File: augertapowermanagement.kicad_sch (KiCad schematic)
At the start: 37 parts, among them J1 5v block, J10 USB_A_Stacked, J11 USB_A_Stacked, J12 USB_A_Stacked, J2 Image shown is a representati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, J3 gnd block, J4 0ZCF0200AF2C, J5 Screw_Terminal_01x10, J6 Screw_Terminal_01x10, J7 Screw_Terminal_01x10, J8 Screw_Terminal_01x08, J9 USB_A_Stacked, K1 J107F1CS203VDC.80, K2 J107F1CS203VDC.80, Q1 2N3904, SW1 SW_SPDT, U1 ESP32-DEVKITC-32D, U2 MCP9808_MSOP, U25 L7812

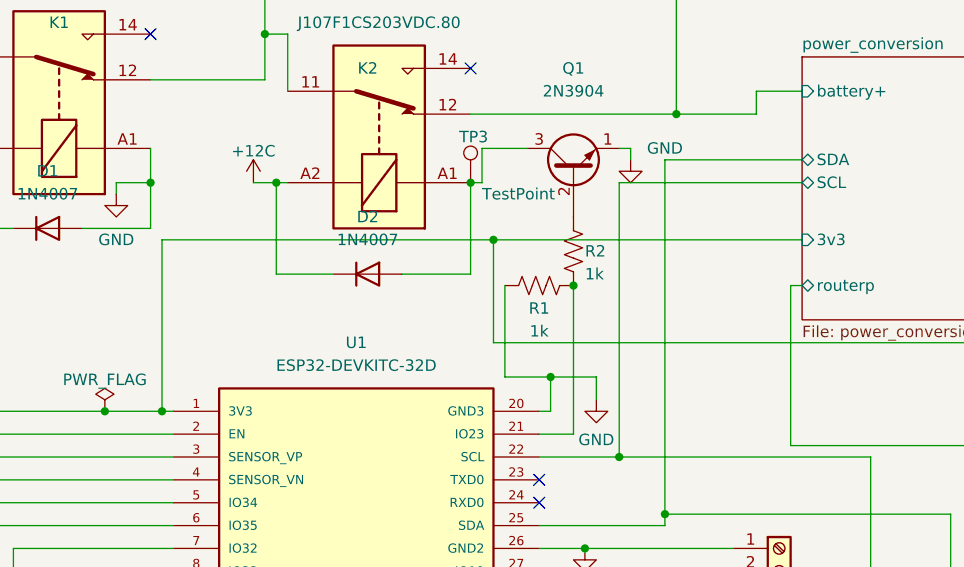
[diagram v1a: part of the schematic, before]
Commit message: fixes
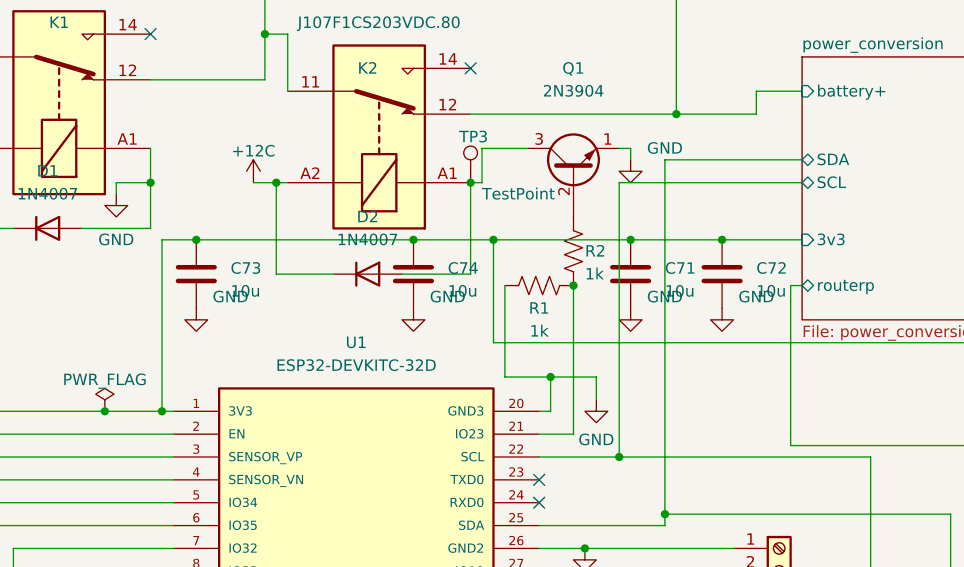
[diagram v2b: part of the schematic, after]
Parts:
- added C71, C72, C73, C74: 10u, Capacitor_SMD:C_1210_3225Metric_Pad1.33x2.70mm_HandSolder, symbol Device:C
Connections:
- net -BATT: now also C71.2, C72.2, C73.2, C74.2
- net power_conversion/3v3: now also C71.1, C72.1, C73.1, C74.1
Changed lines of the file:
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@@
   (junction (at 176.53 101.6) (diameter 0) (color 0 0 0 0)
   )
+  (junction (at 128.27 71.12) (diameter 0) (color 0 0 0 0)
+  )
   (junction (at 45.72 43.18) (diameter 0) (color 0 0 0 0)
   )
@@
   (junction (at 132.08 101.6) (diameter 0) (color 0 0 0 0)
   )
+  (junction (at 138.43 71.12) (diameter 0) (color 0 0 0 0)
+  )
   (junction (at 69.85 90.17) (diameter 0) (color 0 0 0 0)
   )
@@
   (junction (at 54.61 60.96) (diameter 0) (color 0 0 0 0)
   )
+  (junction (at 80.01 71.12) (diameter 0) (color 0 0 0 0)
+  )
   (junction (at 45.72 50.8) (diameter 0) (color 0 0 0 0)
   )
@@
   )
   (junction (at 220.98 93.98) (diameter 0) (color 0 0 0 0)
+  )
+  (junction (at 104.14 71.12) (diameter 0) (color 0 0 0 0)
   )
   (junction (at 29.21 154.94) (diameter 0) (color 0 0 0 0)
@@
     (stroke (width 0) (type default))
   )
-  (wire (pts (xy 76.2 71.12) (xy 113.03 71.12))
+  (wire (pts (xy 76.2 71.12) (xy 80.01 71.12))
     (stroke (width 0) (type default))
   )
@@
     (stroke (width 0) (type default))
   )
+  (wire (pts (xy 128.27 71.12) (xy 138.43 71.12))
+    (stroke (width 0) (type default))
+  )
   (wire (pts (xy 71.12 156.21) (xy 69.85 156.21))
     (stroke (width 0) (type default))
@@
     (stroke (width 0) (type default))
   )
+  (wire (pts (xy 80.01 71.12) (xy 104.14 71.12))
+    (stroke (width 0) (type default))
+  )
   (wire (pts (xy 123.19 144.78) (xy 87.63 144.78))
     (stroke (width 0) (type default))
@@
     (stroke (width 0) (type default))
   )
+  (wire (pts (xy 138.43 71.12) (xy 147.32 71.12))
+    (stroke (width 0) (type default))
+  )
   (wire (pts (xy 118.11 95.25) (xy 127 95.25))
     (stroke (width 0) (type default))
@@
     (stroke (width 0) (type default))
   )
+  (wire (pts (xy 104.14 71.12) (xy 113.03 71.12))
+    (stroke (width 0) (type default))
+  )
   (wire (pts (xy 35.56 148.59) (xy 76.2 148.59))
     (stroke (width 0) (type default))
@@
     (stroke (width 0) (type default))
   )
-  (wire (pts (xy 113.03 71.12) (xy 147.32 71.12))
+  (wire (pts (xy 113.03 71.12) (xy 128.27 71.12))
     (stroke (width 0) (type default))
   )
@@
   (wire (pts (xy 176.53 50.8) (xy 176.53 13.97))
     (stroke (width 0) (type default))
+  )
+  (symbol (lib_id "Device:C") (at 104.14 74.93 0) (unit 1)
+    (in_bom yes) (on_board yes) (dnp no) (fields_autoplaced)
+    (property "Reference" "C74" (at 107.95 74.295 0)
+      (effects (font (size 1.27 1.27)) (justify left))
+    )
+    (property "Value" "10u" (at 107.95 76.835 0)
+      (effects (font (size 1.27 1.27)) (justify left))
+    )
+    (property "Footprint" "Capacitor_SMD:C_1210_3225Metric_Pad1.33x2.70mm_HandSolder" (at 105.1052 78.74 0)
+      (effects (font (size 1.27 1.27)) hide)
+    )
+    (property "Datasheet" "~" (at 104.14 74.93 0)
+      (effects (font (size 1.27 1.27)) hide)
+    )
+    (pin "1")
+    (pin "2")
+    (instances
+      (project "augertapowermanagement"
+        (path "/65134029-dbd2-409a-85a8-13c2a33ff019"
+          (reference "C74") (unit 1)
+        )
+      )
+    )
   )
   (symbol (lib_id "power:GND") (at 43.18 31.75 0) (unit 1)
@@
         (path "/65134029-dbd2-409a-85a8-13c2a33ff019"
           (reference "J2") (unit 1)
+        )
+      )
+    )
+  )
+  (symbol (lib_id "power:GND") (at 104.14 78.74 0) (unit 1)
+    (in_bom yes) (on_board yes) (dnp no)
+    (property "Reference" "#PWR067" (at 104.14 85.09 0)
+      (effects (font (size 1.27 1.27)) hide)
+    )
+    (property "Value" "GND" (at 107.95 77.47 0)
+      (effects (font (size 1.27 1.27)))
+    )
+    (property "Footprint" "" (at 104.14 78.74 0)
+      (effects (font (size 1.27 1.27)) hide)
+    )
+    (property "Datasheet" "" (at 104.14 78.74 0)
+      (effects (font (size 1.27 1.27)) hide)
+    )
+    (pin "1")
+    (instances
+      (project "augertapowermanagement"
+        (path "/65134029-dbd2-409a-85a8-13c2a33ff019"
+          (reference "#PWR067") (unit 1)
         )
       )
@@
         (path "/65134029-dbd2-409a-85a8-13c2a33ff019"
           (reference "J3") (unit 1)
+        )
+      )
+    )
+  )
+  (symbol (lib_id "power:GND") (at 80.01 78.74 0) (unit 1)
+    (in_bom yes) (on_board yes) (dnp no)
+    (property "Reference" "#PWR066" (at 80.01 85.09 0)
+      (effects (font (size 1.27 1.27)) hide)
+    )
+    (property "Value" "GND" (at 83.82 77.47 0)
+      (effects (font (size 1.27 1.27)))
+    )
+    (property "Footprint" "" (at 80.01 78.74 0)
+      (effects (font (size 1.27 1.27)) hide)
+    )
+    (property "Datasheet" "" (at 80.01 78.74 0)
+      (effects (font (size 1.27 1.27)) hide)
+    )
+    (pin "1")
+    (instances
+      (project "augertapowermanagement"
+        (path "/65134029-dbd2-409a-85a8-13c2a33ff019"
+          (reference "#PWR066") (unit 1)
         )
       )
@@
         (path "/65134029-dbd2-409a-85a8-13c2a33ff019"
           (reference "#PWR05") (unit 1)
+        )
+      )
+    )
+  )
+  (symbol (lib_id "Device:C") (at 128.27 74.93 0) (unit 1)
+    (in_bom yes) (on_board yes) (dnp no) (fields_autoplaced)
+    (property "Reference" "C71" (at 132.08 74.295 0)
+      (effects (font (size 1.27 1.27)) (justify left))
+    )
+    (property "Value" "10u" (at 132.08 76.835 0)
+      (effects (font (size 1.27 1.27)) (justify left))
+    )
+    (property "Footprint" "Capacitor_SMD:C_1210_3225Metric_Pad1.33x2.70mm_HandSolder" (at 129.2352 78.74 0)
+      (effects (font (size 1.27 1.27)) hide)
+    )
+    (property "Datasheet" "~" (at 128.27 74.93 0)
+      (effects (font (size 1.27 1.27)) hide)
+    )
+    (pin "1")
+    (pin "2")
+    (instances
+      (project "augertapowermanagement"
+        (path "/65134029-dbd2-409a-85a8-13c2a33ff019"
+          (reference "C71") (unit 1)
         )
       )
@@
     )
   )
+  (symbol (lib_id "Device:C") (at 80.01 74.93 0) (unit 1)
+    (in_bom yes) (on_board yes) (dnp no) (fields_autoplaced)
+    (property "Reference" "C73" (at 83.82 74.295 0)
+      (effects (font (size 1.27 1.27)) (justify left))
+    )
+    (property "Value" "10u" (at 83.82 76.835 0)
+      (effects (font (size 1.27 1.27)) (justify left))
+    )
+    (property "Footprint" "Capacitor_SMD:C_1210_3225Metric_Pad1.33x2.70mm_HandSolder" (at 80.9752 78.74 0)
+      (effects (font (size 1.27 1.27)) hide)
+    )
+    (property "Datasheet" "~" (at 80.01 74.93 0)
+      (effects (font (size 1.27 1.27)) hide)
+    )
+    (pin "1")
+    (pin "2")
+    (instances
+      (project "augertapowermanagement"
+        (path "/65134029-dbd2-409a-85a8-13c2a33ff019"
+          (reference "C73") (unit 1)
+        )
+      )
+    )
+  )
   (symbol (lib_id "Connector:TestPoint") (at 110.49 64.77 0) (unit 1)
     (in_bom yes) (on_board yes) (dnp no)
@@
     )
   )
+  (symbol (lib_id "power:GND") (at 128.27 78.74 0) (unit 1)
+    (in_bom yes) (on_board yes) (dnp no)
+    (property "Reference" "#PWR064" (at 128.27 85.09 0)
+      (effects (font (size 1.27 1.27)) hide)
+    )
+    (property "Value" "GND" (at 132.08 77.47 0)
+      (effects (font (size 1.27 1.27)))
+    )
+    (property "Footprint" "" (at 128.27 78.74 0)
+      (effects (font (size 1.27 1.27)) hide)
+    )
+    (property "Datasheet" "" (at 128.27 78.74 0)
+      (effects (font (size 1.27 1.27)) hide)
+    )
+    (pin "1")
+    (instances
+      (project "augertapowermanagement"
+        (path "/65134029-dbd2-409a-85a8-13c2a33ff019"
+          (reference "#PWR064") (unit 1)
+        )
+      )
+    )
+  )
   (symbol (lib_name "GND_2") (lib_id "power:GND") (at 22.86 60.96 0) (unit 1)
     (in_bom yes) (on_board yes) (dnp no) (fields_autoplaced)
@@
         (path "/65134029-dbd2-409a-85a8-13c2a33ff019"
           (reference "H4") (unit 1)
+        )
+      )
+    )
+  )
+  (symbol (lib_id "power:GND") (at 138.43 78.74 0) (unit 1)
+    (in_bom yes) (on_board yes) (dnp no)
+    (property "Reference" "#PWR065" (at 138.43 85.09 0)
+      (effects (font (size 1.27 1.27)) hide)
+    )
+    (property "Value" "GND" (at 142.24 77.47 0)
+      (effects (font (size 1.27 1.27)))
+    )
+    (property "Footprint" "" (at 138.43 78.74 0)
+      (effects (font (size 1.27 1.27)) hide)
+    )
+    (property "Datasheet" "" (at 138.43 78.74 0)
+      (effects (font (size 1.27 1.27)) hide)
+    )
+    (pin "1")
+    (instances
+      (project "augertapowermanagement"
+        (path "/65134029-dbd2-409a-85a8-13c2a33ff019"
+          (reference "#PWR065") (unit 1)
         )
       )
@@
         )
       )
+    )
+  )
+  (symbol (lib_id "Device:C") (at 138.43 74.93 0) (unit 1)
+    (in_bom yes) (on_board yes) (dnp no) (fields_autoplaced)
+    (property "Reference" "C72" (at 142.24 74.295 0)
+      (effects (font (size 1.27 1.27)) (justify left))
+    )
+    (property "Value" "10u" (at 142.24 76.835 0)
+      (effects (font (size 1.27 1.27)) (justify left))
+    )
+    (property "Footprint" "Capacitor_SMD:C_1210_3225Metric_Pad1.33x2.70mm_HandSolder" (at 139.3952 78.74 0)
+      (effects (font (size 1.27 1.27)) hide)
+    )
+    (property "Datasheet" "~" (at 138.43 74.93 0)
+      (effects (font (size 1.27 1.27)) hide)
+    )
+    (pin "1")
+    (pin "2")
+    (instances
+      (project "augertapowermanagement"
+        (path "/65134029-dbd2-409a-85a8-13c2a33ff019"
+          (reference "C72") (unit 1)
+        )
+      )
